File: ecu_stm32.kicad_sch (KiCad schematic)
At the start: 12 parts, among them J3 ARM Cortex Debug

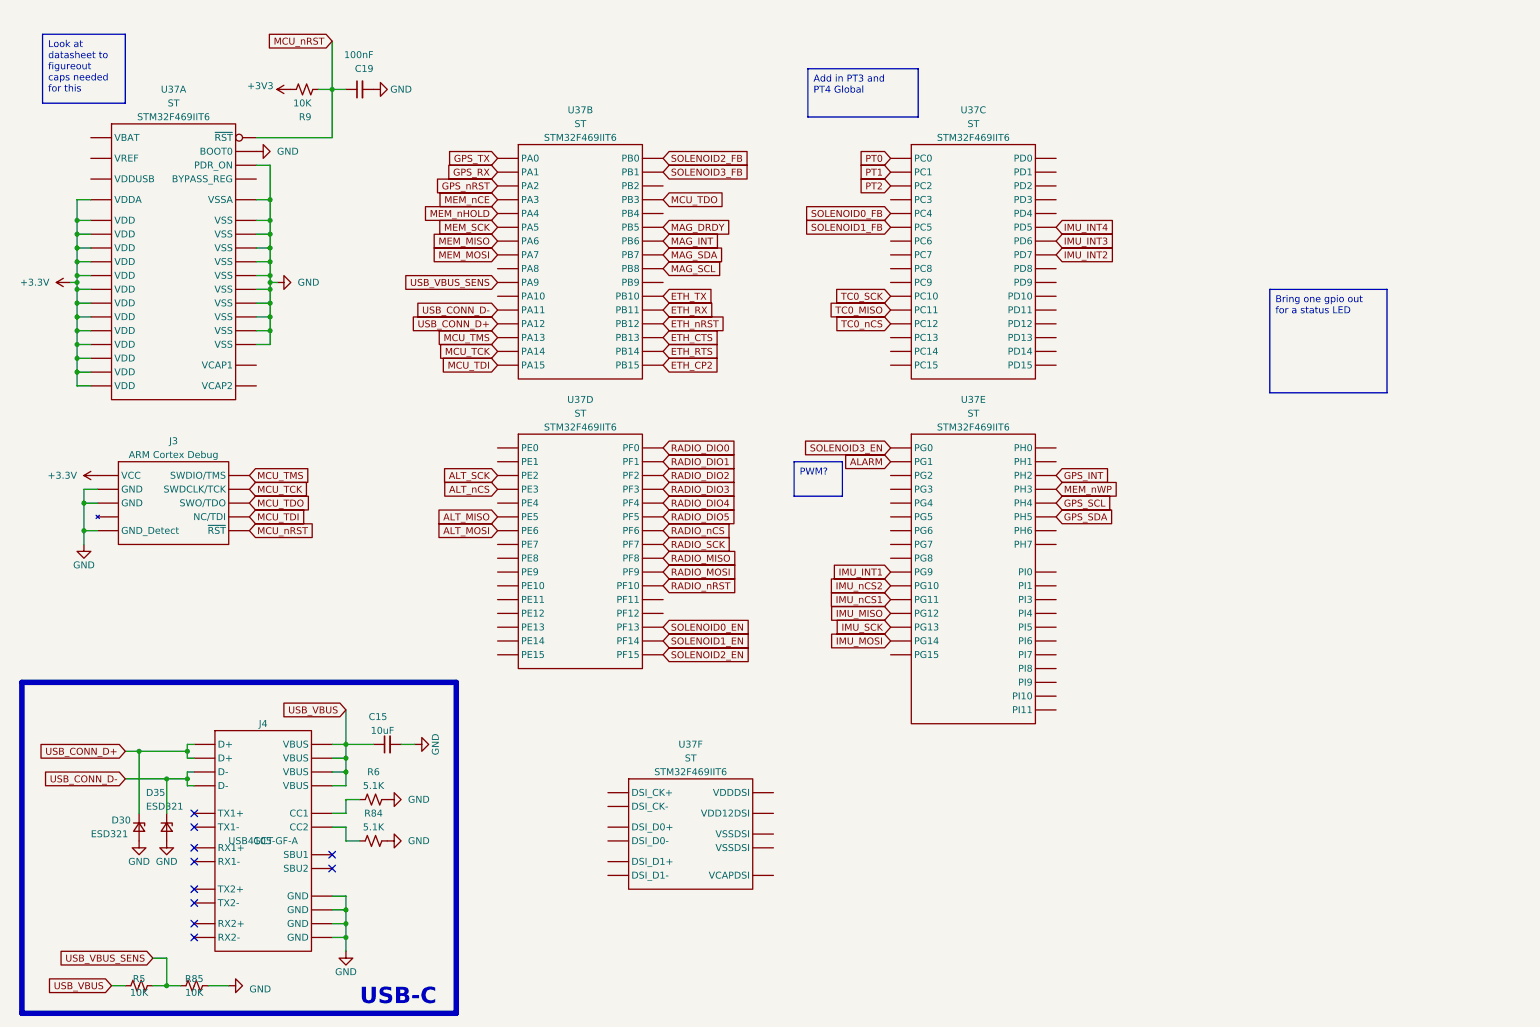
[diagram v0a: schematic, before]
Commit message: added capacitors and resolved all comments
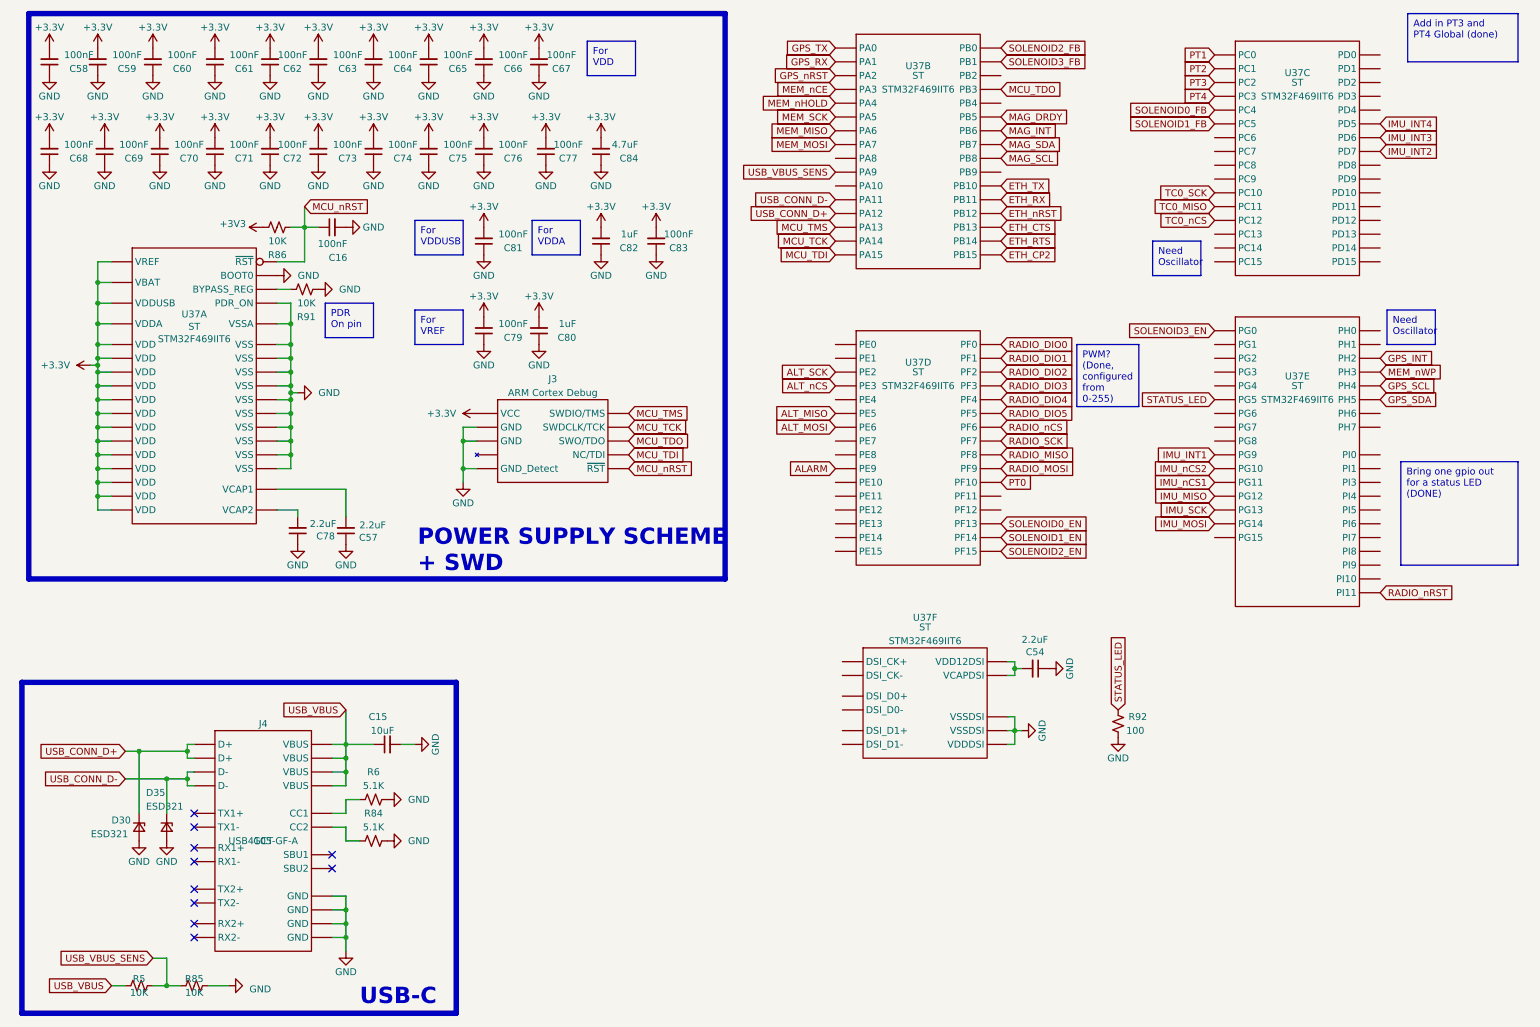
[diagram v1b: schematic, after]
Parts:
- added C54, C57, C78: 2.2uF, Capacitor_SMD:C_0603_1608Metric, symbol Device:C_Small
- added C58, C59, C60, C61, C62, C63, C64, C65, C66, C67, C68, C69, C70, C71, C72, C73, C74, C75, C76, C77, C79, C81, C83: 100nF, Capacitor_SMD:C_0603_1608Metric, symbol Device:C_Small
- added C80, C82: 1uF, Capacitor_SMD:C_0603_1608Metric, symbol Device:C_Small
- added C84: 4.7uF, Capacitor_SMD:C_0603_1608Metric, symbol Device:C_Small
- added R91: 10K, Resistor_SMD:R_0603_1608Metric_Pad0.98x0.95mm_HandSolder, symbol Device:R_Small_US
- added R92: 100, Resistor_SMD:R_0603_1608Metric_Pad0.98x0.95mm_HandSolder, symbol Device:R_Small_US
- renumbered C19 to C16, R9 to R86
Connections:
- net +3.3V: now also U37.118 (VDDUSB), U37.38 (VREF), U37.6 (VBAT), C58.2, C59.2, C60.2, C61.2, C62.2, C63.2, C64.2, C65.2, C66.2, C67.2, C68.2, C69.2, C70.2, C71.2, C72.2, C73.2, C74.2, C75.2, C76.2, C77.2, C79.2, C80.2, C81.2, C82.2, C83.2, C84.2
- net ALARM: now also U37.70 (PE9); no longer U37.67 (PG1)
- net GND: now also U37.103 (VSSDSI), U37.109 (VSSDSI), U37.99 (VDDDSI), C54.1, C57.1, C58.1, C59.1, C60.1, C61.1, C62.1, C63.1, C64.1, C65.1, C66.1, C67.1, C68.1, C69.1, C70.1, C71.1, C72.1, C73.1, C74.1, C75.1, C76.1, C77.1, C78.1, C79.1, C80.1, C81.1, C82.1, C83.1, C84.1, R91.2, R92.1
- net PT0: now also U37.28 (PF10); no longer U37.32 (PC0)
- net PT1: now also U37.32 (PC0); no longer U37.33 (PC1)
- net PT2: now also U37.33 (PC1); no longer U37.34 (PC2)
- net RADIO_nRST: now also U37.13 (PI11); no longer U37.28 (PF10)
- net PT4: now reaches U37.35 (PC3)
- net at U37.129 (VCAP2): now also C78.2
- net at U37.48 (BYPASS_REG): now also R91.1
- net at U37.81 (VCAP1): now also C57.2
- net at U37.100 (VCAPDSI): now also U37.106 (VDD12DSI), C54.2
- net STATUS_LED: now reaches U37.113 (PG5)
- net STATUS_LED: now also R92.2
- new net PT3: U37.34 (PC2)
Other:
- note added: "POWER SUPPLY SCHEME + SWD"
- moved on the sheet: C16, J3, R86, U37A, U37B, U37C, U37D, U37E, U37F
